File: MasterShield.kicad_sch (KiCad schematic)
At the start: 67 parts, among them J1 CONTROL/SERIAL, J2 MISC, J3 ADC/SENSE, J4 POWER, J5 RS485 A, J6 EXTRA POWER, J7 BATT, J8 RS485 B, J9 BYPASS, Q1 S8050, Q2 Si9945AEY-T1, Q3 S8050, U1 MAX485E, U2 BTS724G, U3 74LVC1G08GW, U4 LM321, U5 LM2596S-5, U6 LTC4365TS8

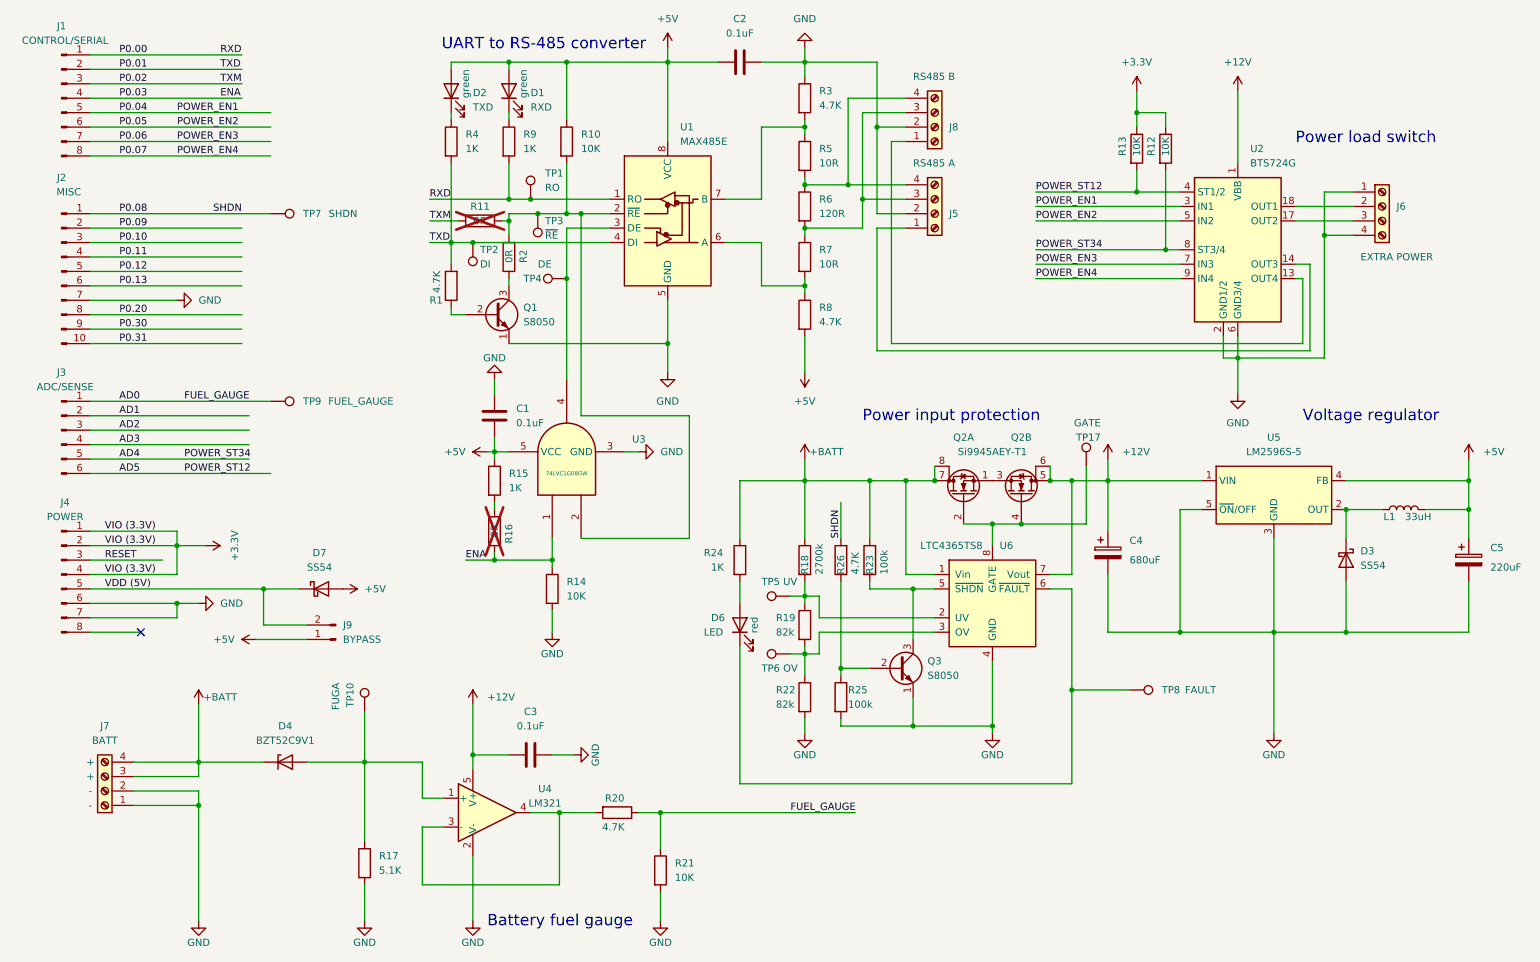
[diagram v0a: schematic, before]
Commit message: ...
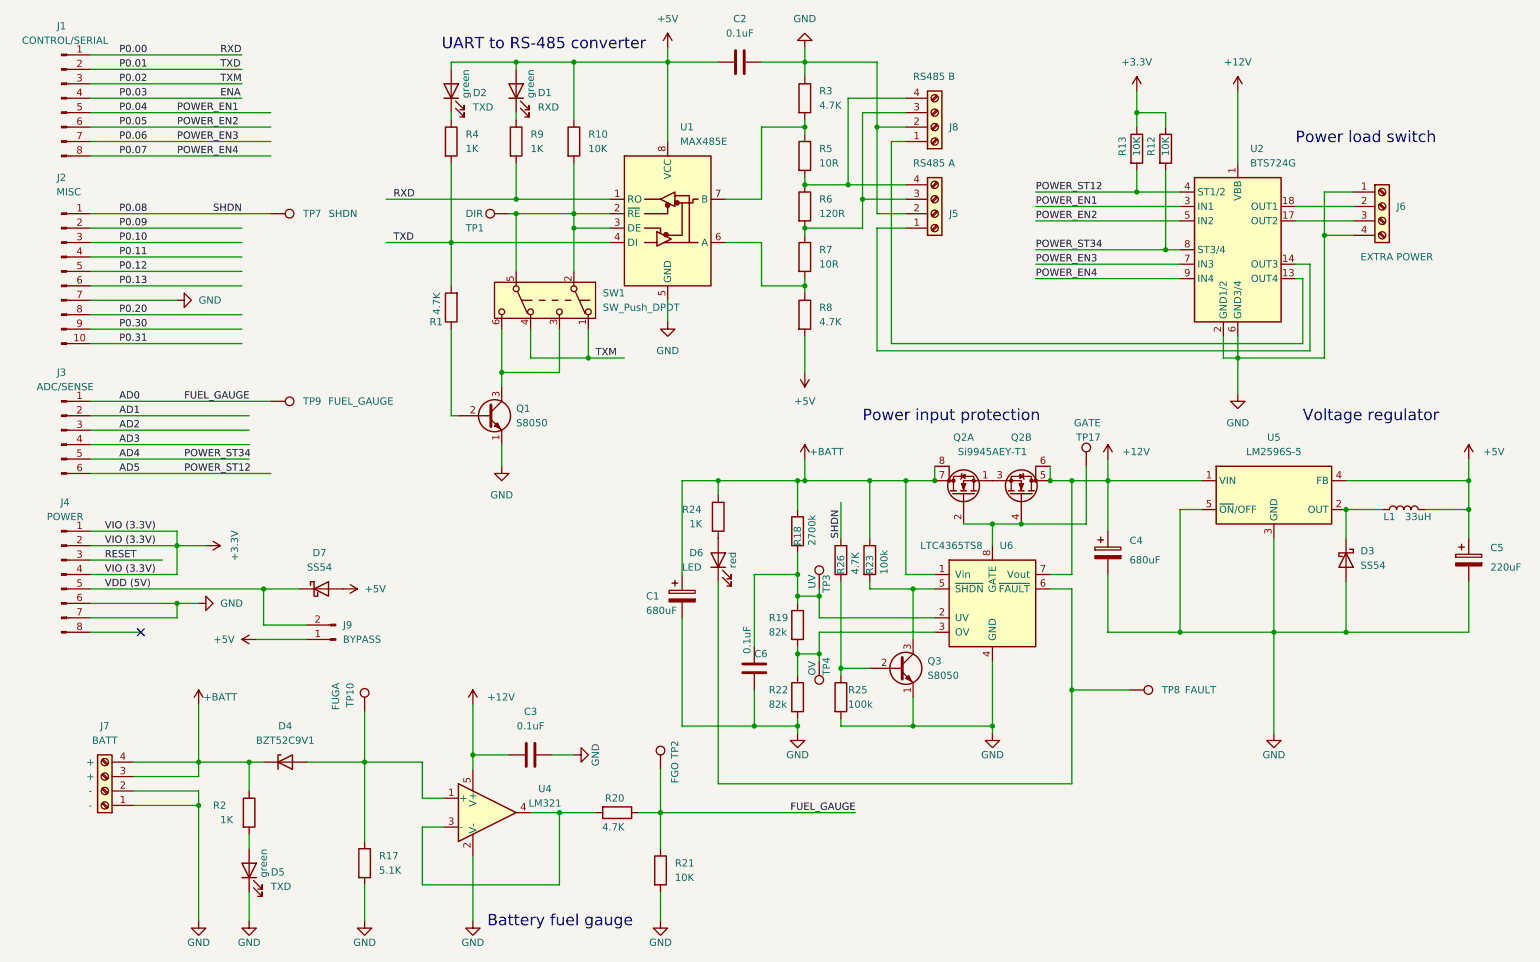
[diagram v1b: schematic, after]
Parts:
- removed C1: 0.1uF, Capacitor_SMD:C_0805_2012Metric, symbol Device:C
- removed R11, R16: 0R, Resistor_SMD:R_0805_2012Metric, symbol Device:R
- removed R14: 10K, Resistor_SMD:R_0805_2012Metric, symbol Device:R
- removed R15: 1K, Resistor_SMD:R_0805_2012Metric, symbol Device:R
- removed TP5: UV, TestPoint:TestPoint_Pad_D2.0mm, symbol Connector:TestPoint
- removed TP6: OV, TestPoint:TestPoint_Pad_D2.0mm, symbol Connector:TestPoint
- removed U3: 74LVC1G08GW, Package_TO_SOT_SMD:SOT-353_SC-70-5, symbol 74xGxx:74AUC1G08
- added C1: 680uF, Capacitor_SMD:CP_Elec_10x10.5, symbol Device:C_Polarized
- added C6: 0.1uF, Capacitor_SMD:C_0805_2012Metric, symbol Device:C
- added D5: TXD, LED_SMD:LED_0805_2012Metric, symbol Device:LED
- added SW1: SW_Push_DPDT, Button_Switch_SMD:Nidec_Copal_SH-7010A, symbol Switch:SW_Push_DPDT
- R2: value 0R -> 1K; LCSC C17477 -> C17513
- TP1: value RO -> DIR
- TP2: value DI -> FGO
- TP3: value ~{RE} -> UV
- TP4: value DE -> OV
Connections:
- net +BATT: now also R2.1, C1.1
- net AD0: now also TP2.1
- net GND: now also C1.2, C6.1, D5.1 (K)
- net P0.00: no longer TP1.1
- net P0.01: no longer TP2.1
- net P0.02: now also SW1.1 (A), SW1.4 (A)
- net at R18.2, R19.1, U6.2 (UV): now also TP3.1, C6.2
- net at R19.2, R22.1, U6.3 (OV): now also TP4.1
- net at R10.2, U1.2 (~{RE}): now also TP1.1, U1.3 (DE), SW1.2 (B), SW1.5 (B); no longer R2.2, TP3.1
- net at Q1.3 (C): now also SW1.3 (C), SW1.6 (C); no longer R2.1
- new net: D5.2 (A), R2.2
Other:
- moved on the sheet: D1, D6, Q1, R1, R10, R18, R19, R22, R24, R9
